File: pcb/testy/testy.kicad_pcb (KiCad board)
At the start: 2 copper layers, 114.5 x 101.4 mm, 94 parts, among them P1 OLED, P2 ICSP, SW0:0 SW_Push, SW0:1 SW_Push, SW0:2 SW_Push, SW0:3 SW_Push, SW0:4 SW_Push, SW1:0 SW_Push, SW1:1 SW_Push, SW1:2 SW_Push, SW1:3 SW_Push, SW1:4 SW_Push, SW2:0 SW_Push, SW2:1 SW_Push, SW2:2 SW_Push, SW2:3 SW_Push, SW2:4 SW_Push, SW3:0 SW_Push, SW3:1 SW_Push, SW3:2 SW_Push, SW3:3 SW_Push, SW3:4 SW_Push, SW3:5 SW_Push, SW4:1 SW_Push, SW4:2 SW_Push, SW4:3 SW_Push, SW4:4 SW_Push, SW4:5 SW_Push

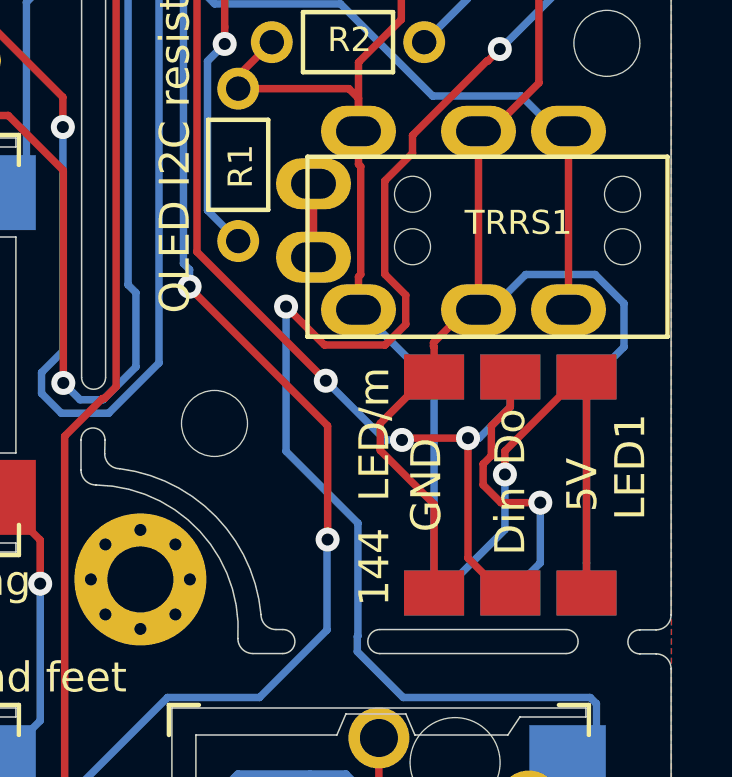
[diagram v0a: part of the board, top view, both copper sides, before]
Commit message: fix: undo some wrong decisions with the LEDs
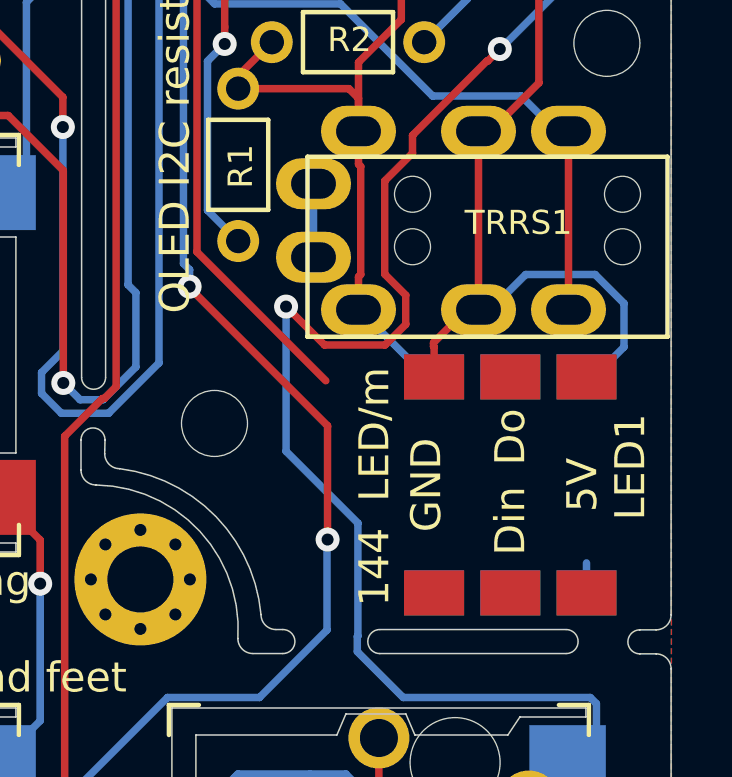
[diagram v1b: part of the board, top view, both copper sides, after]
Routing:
- net VCC: track 85.1 -> 61.1 mm, vias 3 -> 2
- net GND: track 238.3 -> 223.2 mm
- net LED: track 71.8 -> 57.4 mm, vias 3 -> 0
- net Net-(LED1-Pad1): track 9.55 -> 0.00 mm, vias 1 -> 0
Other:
- board text added: "TODO add extra data pin so we can handwire LEDs over the TRRS cable"
- board text added: "TODO don't directly connect the halves on the connector"
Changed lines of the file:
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@@
   (general
     (thickness 1.6)
-    (drawings 1027)
-    (tracks 1410)
+    (drawings 1029)
+    (tracks 1372)
     (zones 0)
     (modules 94)
@@
     (pad 1 thru_hole circle (at 1.166726 -1.166726 270) (size 0.7 0.7) (drill 0.4) (layers *.Cu *.Mask))
   )
+  (gr_text "TODO add extra data pin so we can\nhandwire LEDs over the TRRS cable" (at 201.83 107.7) (layer Dwgs.User)
+    (effects (font (size 1 1) (thickness 0.15)))
+  )
+  (gr_text "TODO don't directly connect the halves on the connector" (at 209.74 103.79) (layer Dwgs.User)
+    (effects (font (size 1 1) (thickness 0.15)))
+  )
   (gr_text "OLED I2C resistors" (at 170.4 90.3 90) (layer F.SilkS)
     (effects (font (size 1 1) (thickness 0.15)))
@@
   (segment (start 181.51 80.97212) (end 182.16106 80.32106) (width 0.25) (layer F.Cu) (net 5))
   (segment (start 181.51 81.53962) (end 181.51 80.97212) (width 0.25) (layer F.Cu) (net 5))
-  (segment (start 184.12 104.99) (end 184.12 98.79) (width 0.25) (layer B.Cu) (net 5))
   (segment (start 184.12 105.99) (end 184.12 104.99) (width 0.25) (layer B.Cu) (net 5))
   (segment (start 179.04 98.79) (end 179.04 97.79) (width 0.25) (layer F.Cu) (net 5))
-  (segment (start 178.79 98.79) (end 179.04 98.79) (width 0.25) (layer F.Cu) (net 5))
-  (segment (start 177.244999 100.335001) (end 178.79 98.79) (width 0.25) (layer F.Cu) (net 5))
-  (segment (start 177.244999 101.238001) (end 177.244999 100.335001) (width 0.25) (layer F.Cu) (net 5))
-  (segment (start 179.04 103.033002) (end 177.244999 101.238001) (width 0.25) (layer F.Cu) (net 5))
-  (segment (start 179.04 105.99) (end 179.04 103.033002) (width 0.25) (layer F.Cu) (net 5))
   (via (at 173.03 61.7) (size 0.8) (drill 0.4) (layers F.Cu B.Cu) (net 5))
   (segment (start 178.480001 53.349999) (end 179.33 52.5) (width 0.25) (layer F.Cu) (net 5))
@@
   (segment (start 178.96 80.97212) (end 178.35394 80.36606) (width 0.25) (layer F.Cu) (net 8))
   (segment (start 178.35394 80.36606) (end 175.45 77.46212) (width 0.25) (layer F.Cu) (net 8))
-  (segment (start 179.04 105.99) (end 179.04 98.79) (width 0.25) (layer B.Cu) (net 8))
-  (via (at 181.4 102.04) (size 0.8) (drill 0.4) (layers F.Cu B.Cu) (net 8))
-  (segment (start 181.4 101.26) (end 181.4 102.04) (width 0.25) (layer F.Cu) (net 8))
-  (segment (start 184.12 98.79) (end 183.87 98.79) (width 0.25) (layer F.Cu) (net 8))
-  (segment (start 183.87 98.79) (end 181.4 101.26) (width 0.25) (layer F.Cu) (net 8))
-  (segment (start 179.29 105.99) (end 179.04 105.99) (width 0.25) (layer B.Cu) (net 8))
-  (segment (start 181.4 103.88) (end 179.29 105.99) (width 0.25) (layer B.Cu) (net 8))
-  (segment (start 181.4 102.04) (end 181.4 103.88) (width 0.25) (layer B.Cu) (net 8))
-  (segment (start 184.12 105.99) (end 184.12 98.79) (width 0.25) (layer F.Cu) (net 8))
   (segment (start 176.55 96.55) (end 176.52 96.55) (width 0.25) (layer B.Cu) (net 8))
   (segment (start 178.79 98.79) (end 176.55 96.55) (width 0.25) (layer B.Cu) (net 8))
@@
   (segment (start 176.52 88.305218) (end 177.946499 86.878719) (width 0.25) (layer F.Cu) (net 8))
   (segment (start 176.52 90.6) (end 176.52 88.305218) (width 0.25) (layer F.Cu) (net 8))
-  (segment (start 175.02 94.8) (end 175.02 92.35) (width 0.25) (layer F.Cu) (net 9))
+  (segment (start 175.02 92.35) (end 175.02 94.8) (width 0.25) (layer B.Cu) (net 9))
   (segment (start 93.17 83.145) (end 93.175 83.15) (width 0.25) (layer F.Cu) (net 10))
   (segment (start 93.175 83.15) (end 108.1 83.15) (width 0.25) (layer F.Cu) (net 10))
@@
   (segment (start 180.84 79.07) (end 180.84 78.504315) (width 0.25) (layer F.Cu) (net 45))
   (segment (start 180.84 78.504315) (end 178.84135 76.505665) (width 0.25) (layer F.Cu) (net 45))
-  (segment (start 180.54 100.83) (end 180.17 100.83) (width 0.25) (layer B.Cu) (net 46))
-  (via (at 180.17 100.83) (size 0.8) (drill 0.4) (layers F.Cu B.Cu) (net 46))
-  (segment (start 181.58 98.79) (end 181.58 99.79) (width 0.25) (layer B.Cu) (net 46))
-  (segment (start 181.58 99.79) (end 180.54 100.83) (width 0.25) (layer B.Cu) (net 46))
-  (segment (start 181.33 105.99) (end 181.58 105.99) (width 0.25) (layer F.Cu) (net 46))
-  (segment (start 180.17 104.83) (end 181.33 105.99) (width 0.25) (layer F.Cu) (net 46))
-  (segment (start 180.17 100.83) (end 180.17 104.83) (width 0.25) (layer F.Cu) (net 46))
-  (via (at 177.97 100.89) (size 0.8) (drill 0.4) (layers F.Cu B.Cu) (net 46))
-  (segment (start 180.17 100.83) (end 178.03 100.83) (width 0.25) (layer F.Cu) (net 46))
-  (segment (start 178.03 100.83) (end 177.97 100.89) (width 0.25) (layer F.Cu) (net 46))
-  (segment (start 177.404315 100.89) (end 175.43 98.915685) (width 0.25) (layer B.Cu) (net 46))
-  (segment (start 177.97 100.89) (end 177.404315 100.89) (width 0.25) (layer B.Cu) (net 46))
-  (via (at 175.43 98.915685) (size 0.8) (drill 0.4) (layers F.Cu B.Cu) (net 46))
   (segment (start 184.403701 52.510299) (end 185.28 51.634) (width 0.25) (layer F.Cu) (net 46))
   (segment (start 184.078699 52.835301) (end 184.403701 52.510299) (width 0.25) (layer F.Cu) (net 46))
@@
   (segment (start 173.89 82.54038) (end 173.9 82.53038) (width 0.25) (layer B.Cu) (net 50))
   (segment (start 173.89 84.88) (end 173.89 82.54038) (width 0.25) (layer B.Cu) (net 50))
-  (via (at 182.58 102.98) (size 0.8) (drill 0.4) (layers F.Cu B.Cu) (net 54))
-  (segment (start 181.58 98.79) (end 181.58 99.79) (width 0.25) (layer F.Cu) (net 54))
-  (segment (start 181.266998 102.98) (end 182.58 102.98) (width 0.25) (layer F.Cu) (net 54))
-  (segment (start 181.58 99.79) (end 180.94999 100.42001) (width 0.25) (layer F.Cu) (net 54))
-  (segment (start 180.94999 100.42001) (end 180.94999 101.417008) (width 0.25) (layer F.Cu) (net 54))
-  (segment (start 180.674999 102.388001) (end 181.266998 102.98) (width 0.25) (layer F.Cu) (net 54))
-  (segment (start 180.674999 101.691999) (end 180.674999 102.388001) (width 0.25) (layer F.Cu) (net 54))
-  (segment (start 180.94999 101.417008) (end 180.674999 101.691999) (width 0.25) (layer F.Cu) (net 54))
-  (segment (start 182.58 104.99) (end 181.58 105.99) (width 0.25) (layer B.Cu) (net 54))
-  (segment (start 182.58 102.98) (end 182.58 104.99) (width 0.25) (layer B.Cu) (net 54))
   (zone (net 0) (net_name "") (layer B.Cu) (hatch edge 0.508)
     (connect_pads (clearance 0.508))
